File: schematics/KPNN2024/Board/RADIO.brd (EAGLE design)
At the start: 68.2 x 68.2 mm, 7 parts, among them J1 U.FL-R-SMT-1_10_, J2 U.FL-R-SMT-1_10_

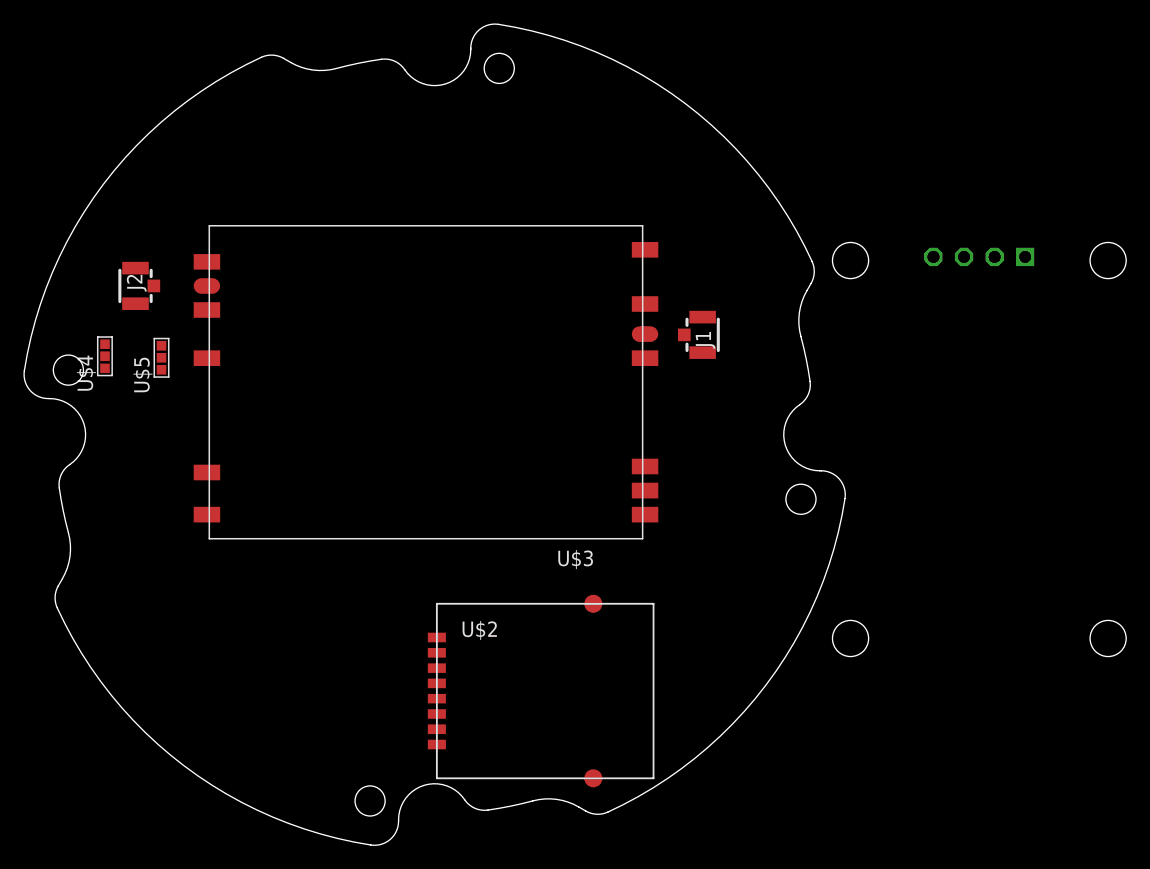
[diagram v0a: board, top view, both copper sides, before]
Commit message: SUS
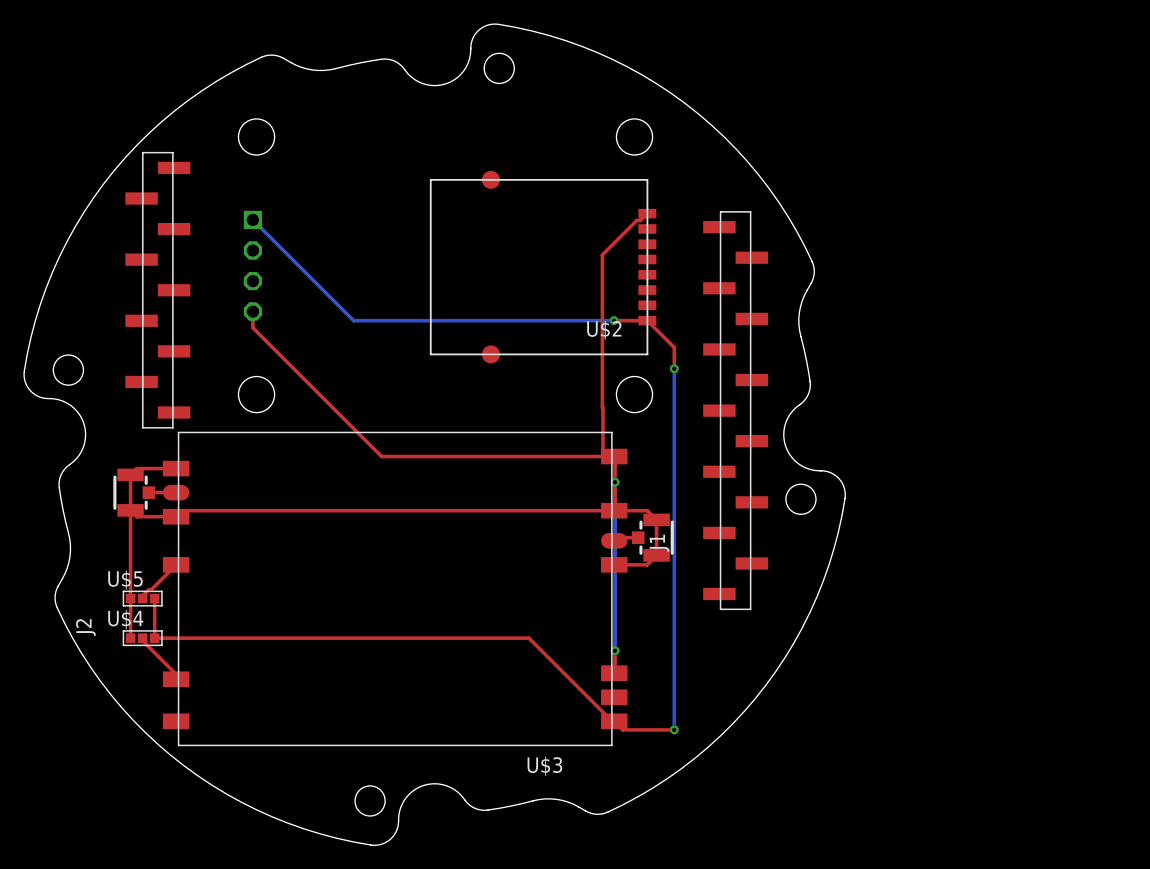
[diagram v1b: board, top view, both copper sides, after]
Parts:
- added U$6: PBS_SMD_X13, UNKNOWN-2024:PBD_SMD_X13
- added U$7: PBS_SMD_X9, UNKNOWN-2024:PBS_SMD_X9
- moved U$1 46.9 mm to (50.9, 64.0), turned to 270 degrees
- moved U$2 35.2 mm to (58.7, 63.9), turned to 180 degrees
- moved U$4 23.6 mm to (25.7, 33.1), turned to 0 degrees
- moved U$5 20.1 mm to (25.7, 36.4), turned to 0 degrees
- moved U$3 17.4 mm to (46.7, 37.2)
- moved J1 17.3 mm to (68.4, 41.4)
- moved J2 17.2 mm to (24.7, 45.2)
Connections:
- new net ADC_FOTO: U$6.10
- new net CE_RADIO: U$7.1
- new net CS_RADIO: U$7.2
- new net DIR_DRIVER: U$6.1
- new net IRQ_RADIO: U$7.3
- new net LATCH_SR: U$6.5
- new net MISO_RADIO: U$7.5
- new net MISO_SR: U$6.8
- new net MOSI_RADIO: U$7.4
- new net MOSI_SR: U$6.9
- new net OE_SR: U$6.6
- new net RX1_BLE: U$6.4
- new net RX2_GPS: U$7.8
- new net SCK_RADIO: U$7.6
- new net SCK_SR: U$6.7
- new net STEP_DRIVER: U$6.2
- new net SV: U$6.11
- new net SW_WMP: U$7.9
- new net TX1_BLE: U$6.3
- new net TX2_GPS: U$7.7
- net 3V3: now also U$6.13
- net GND: now also U$6.12
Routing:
- net GND: track 0.00 -> 147.0 mm, vias 0 -> 2
- net 3V3: track 0.00 -> 120.8 mm, vias 0 -> 3
- net LED1: track 0.00 -> 4.66 mm
- net LED2: track 0.00 -> 4.07 mm
- net ATN_RADIO: track 0.00 -> 2.26 mm
- net RF-IN: track 0.00 -> 2.10 mm
